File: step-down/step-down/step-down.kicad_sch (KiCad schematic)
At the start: 21 parts, among them J0 1725656, J1 1725656, M1 IRF7413ZPBF, M2 IRF7413ZPBF, U1 LTC3807EFE-TRPBF

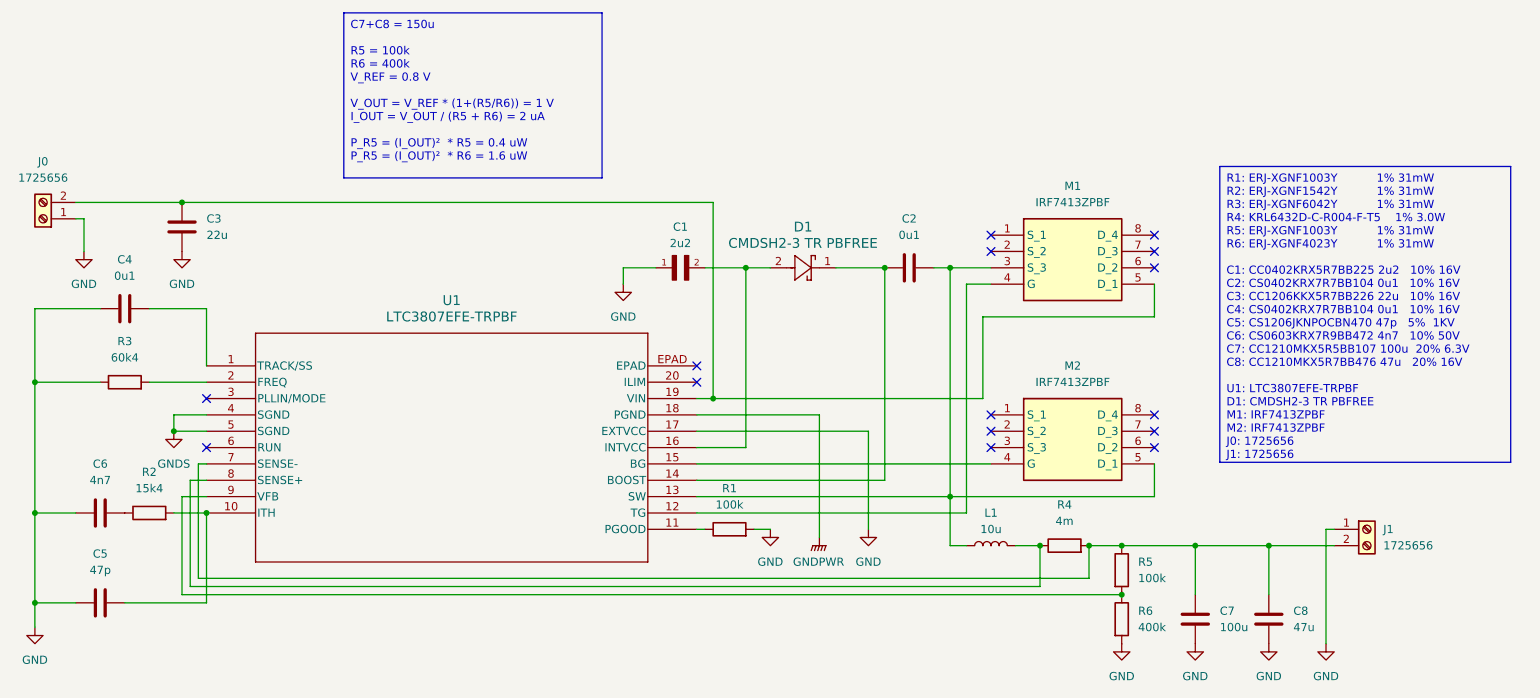
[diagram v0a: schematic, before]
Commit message: v1.1
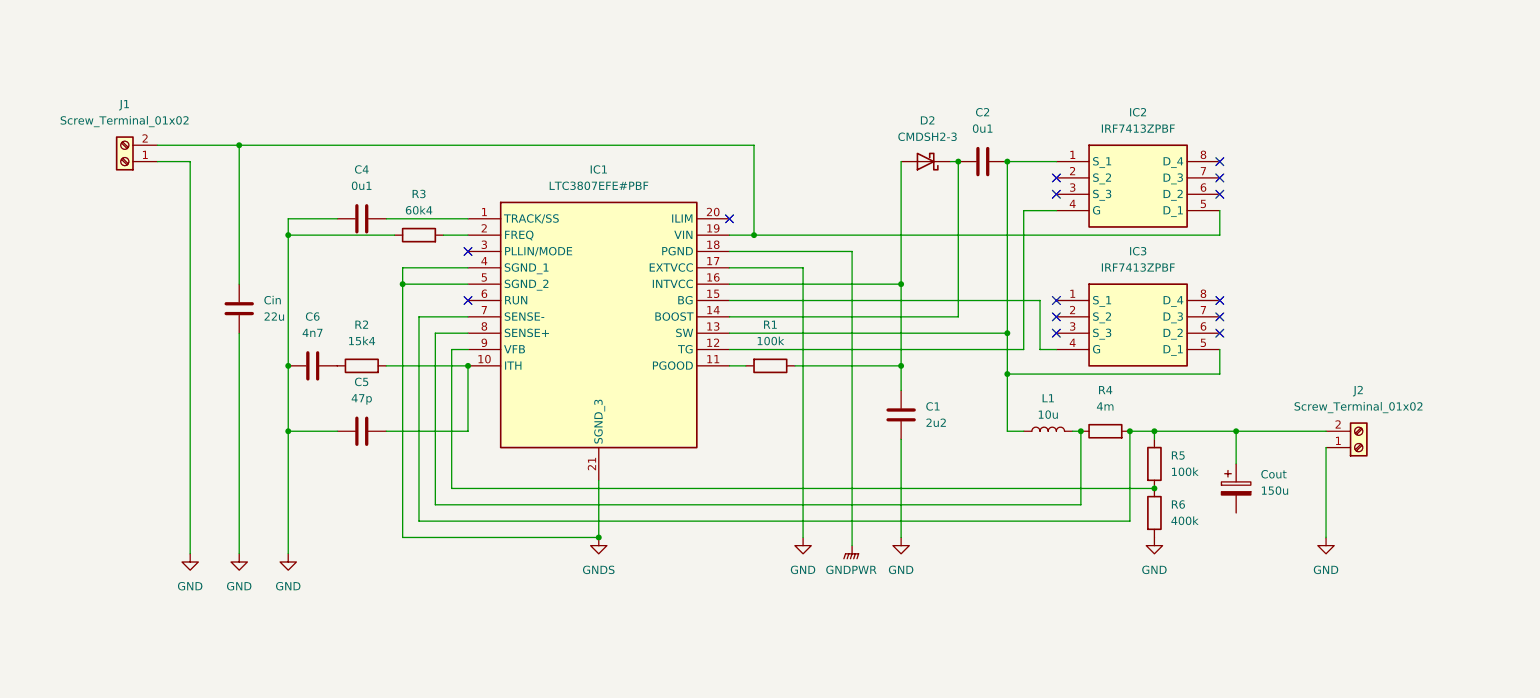
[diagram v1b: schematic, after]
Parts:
- removed C1: 2u2, CC0402KRX5R7BB225:CAPC1005X55N, symbol CC0402KRX5R7BB225:CC0402KRX5R7BB225
- removed C3: 22u, Capacitor_SMD:C_1206_3216Metric, symbol Device:C
- removed C7: 100u, Capacitor_SMD:C_1210_3225Metric, symbol Device:C
- removed C8: 47u, Capacitor_SMD:C_1210_3225Metric, symbol Device:C
- removed D1: CMDSH2-3 TR PBFREE, SDO_CMDSH2-3 TR PBFREE_CNS, symbol 2025-02-07_10-12-59:CMDSH2-3_TR_PBFREE
- removed J0: 1725656, TerminalBlock_Phoenix:TerminalBlock_Phoenix_MKDS-1,5-2-5.08_1x02_P5.08mm_Horizontal, symbol Connector:Screw_Terminal_01x02
- removed M1, M2: IRF7413ZPBF, footprint-libraries:SOIC127P600X175-8N, symbol IRF7413ZPBF:IRF7413ZPBF
- removed U1: LTC3807EFE-TRPBF, TSSOP-20_FE/CB_LIT, symbol LTC3807EFE-TRPBF:LTC3807EFE-TRPBF
- added C1: 2u2, footprints:CC0402KRX5R7BB225, symbol Device:C
- added Cin: 22u, symbol Device:C
- added Cout: 150u, footprints:TAZH157J010LBSZ0H00, symbol Device:C_Polarized
- added D2: CMDSH2-3, footprints:CMDSH2-3_TR_PBFREE, symbol Device:D_Schottky
- added IC1: LTC3807EFE#PBF, SOP65P640X120-21N, symbol LTC3807EFE#PBF:LTC3807EFE#PBF
- added IC2, IC3: IRF7413ZPBF, SOIC127P600X175-8N, symbol IRF7413ZPBF:IRF7413ZPBF
- added J2: Screw_Terminal_01x02, footprints:1725656, symbol Connector:Screw_Terminal_01x02
- C2, C4: footprint Capacitor_SMD:C_0402_1005Metric -> footprints:CAP_CS0402_YAG
- C5: footprint Capacitor_SMD:C_0805_2012Metric -> footprints:CAP_CS1206_YAG
- C6: footprint Capacitor_SMD:C_0603_1608Metric -> footprints:CAP_CS0603_YAG
- J1: value 1725656 -> Screw_Terminal_01x02; footprint TerminalBlock_Phoenix:TerminalBlock_Phoenix_MKDS-1,5-2-5.08_1x02_P5.08mm_Horizontal -> footprints:1725656
- L1: footprint Inductor_SMD:L_Bourns_SRP6060FA -> footprints:AISC-1008F-100G-T
- R1, R5: footprint footprint-libraries:RES_ERJXGNF1003Y -> footprints:ERJ-XGNF1003Y
- R2: footprint footprint-libraries:RES_ERJXGNF1542Y -> footprints:ERJ-XGNF1542Y
- R3: footprint footprint-libraries:RES_ERJXGNF6042Y -> footprints:ERJ-XGNF6042Y
- R4: footprint footprint-libraries:RESC310X630X70N -> footprints:KRL6432D-C-R004-F-T5
- R6: footprint footprint-libraries:RES_ERJXGNF4023Y -> footprints:ERJ-XGNF4023Y
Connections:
- net GND: now also C5.2, C1.2, Cin.2, IC1.17 (EXTVCC), J2.1 (Pin_1); no longer C5.1, R1.2
- net GNDPWR: now also IC1.18 (PGND)
- net GNDS: now also IC1.21 (SGND_3), IC1.4 (SGND_1), IC1.5 (SGND_2)
- net at L1.1: now also C2.2, IC1.13 (SW), IC2.1 (S_1), IC3.5 (D_1); no longer C2.1
- net at R2.2: now also C5.1, IC1.10 (ITH); no longer C5.2
- net at C4.2: now also IC1.1 (TRACK/SS)
- net at R5.2, R6.1: now also IC1.9 (VFB)
- net at L1.2, R4.1: now also IC1.8 (SENSE+)
- net at R4.2, R5.1: now also Cout.1, IC1.7 (SENSE-), J2.2 (Pin_2); no longer J1.2 (Pin_2)
- net at R3.2: now also IC1.2 (FREQ)
- net at R1.1: now also C1.1, D2.2 (A), IC1.16 (INTVCC)
- new net: Cin.1, IC1.19 (VIN), IC2.5 (D_1), J1.2 (Pin_2)
- new net: IC1.11 (PGOOD), R1.2
- new net: IC1.15 (BG), IC3.4 (G)
- new net: C2.1, D2.1 (K), IC1.14 (BOOST)
- new net: IC1.12 (TG), IC2.4 (G)
- no-connect marks 15 -> 14
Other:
- title: Step-down converter -> Step-Down Converter
